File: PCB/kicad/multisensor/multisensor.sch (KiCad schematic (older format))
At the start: 27 parts

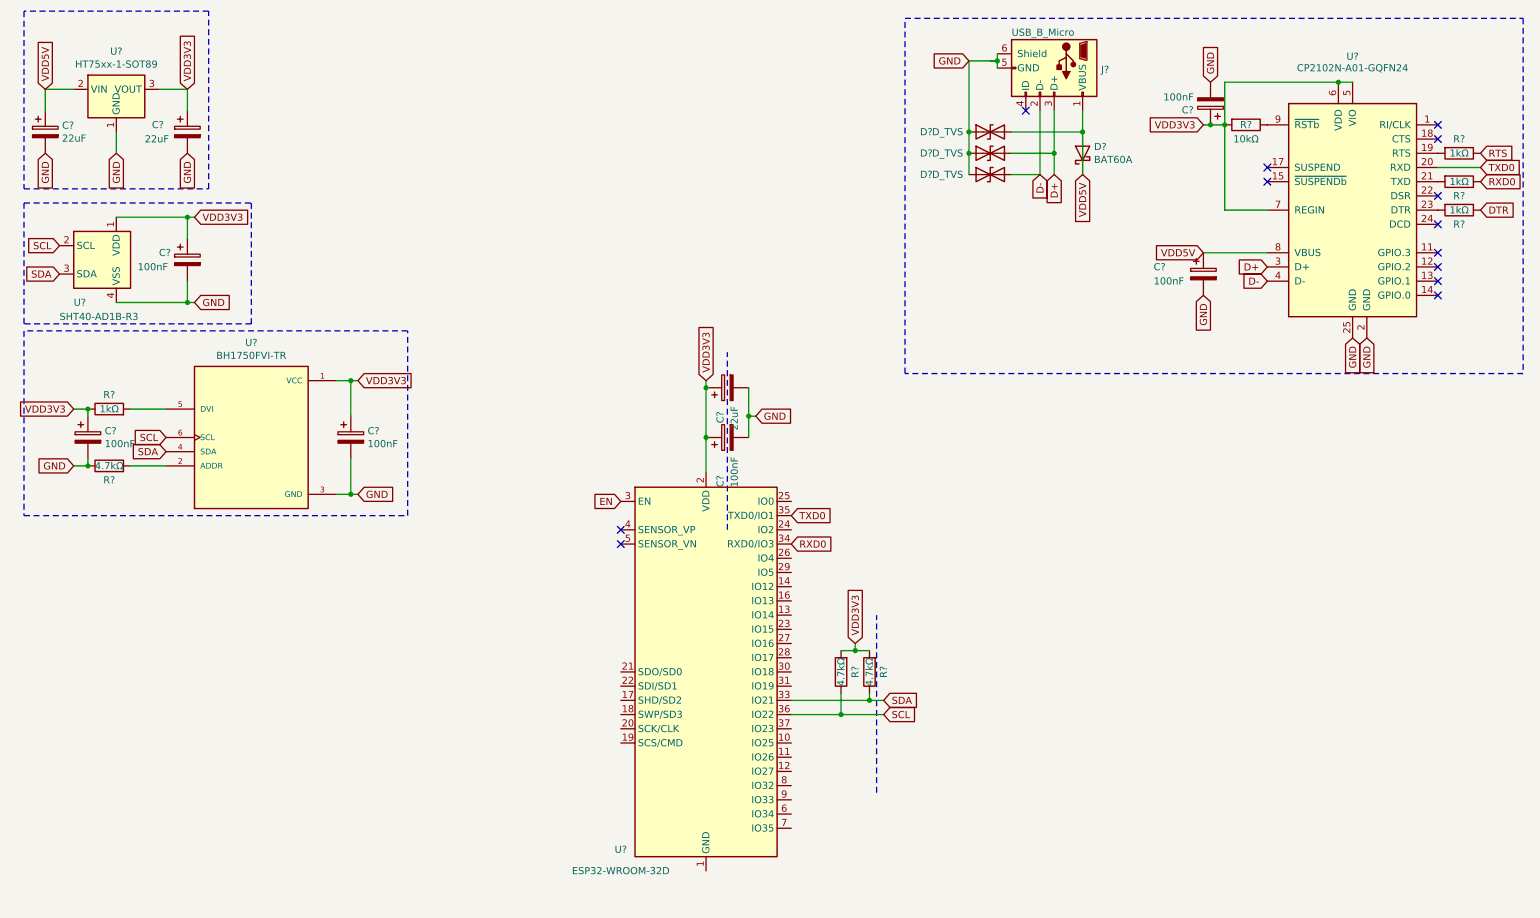
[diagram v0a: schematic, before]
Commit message: pogrammable part USB
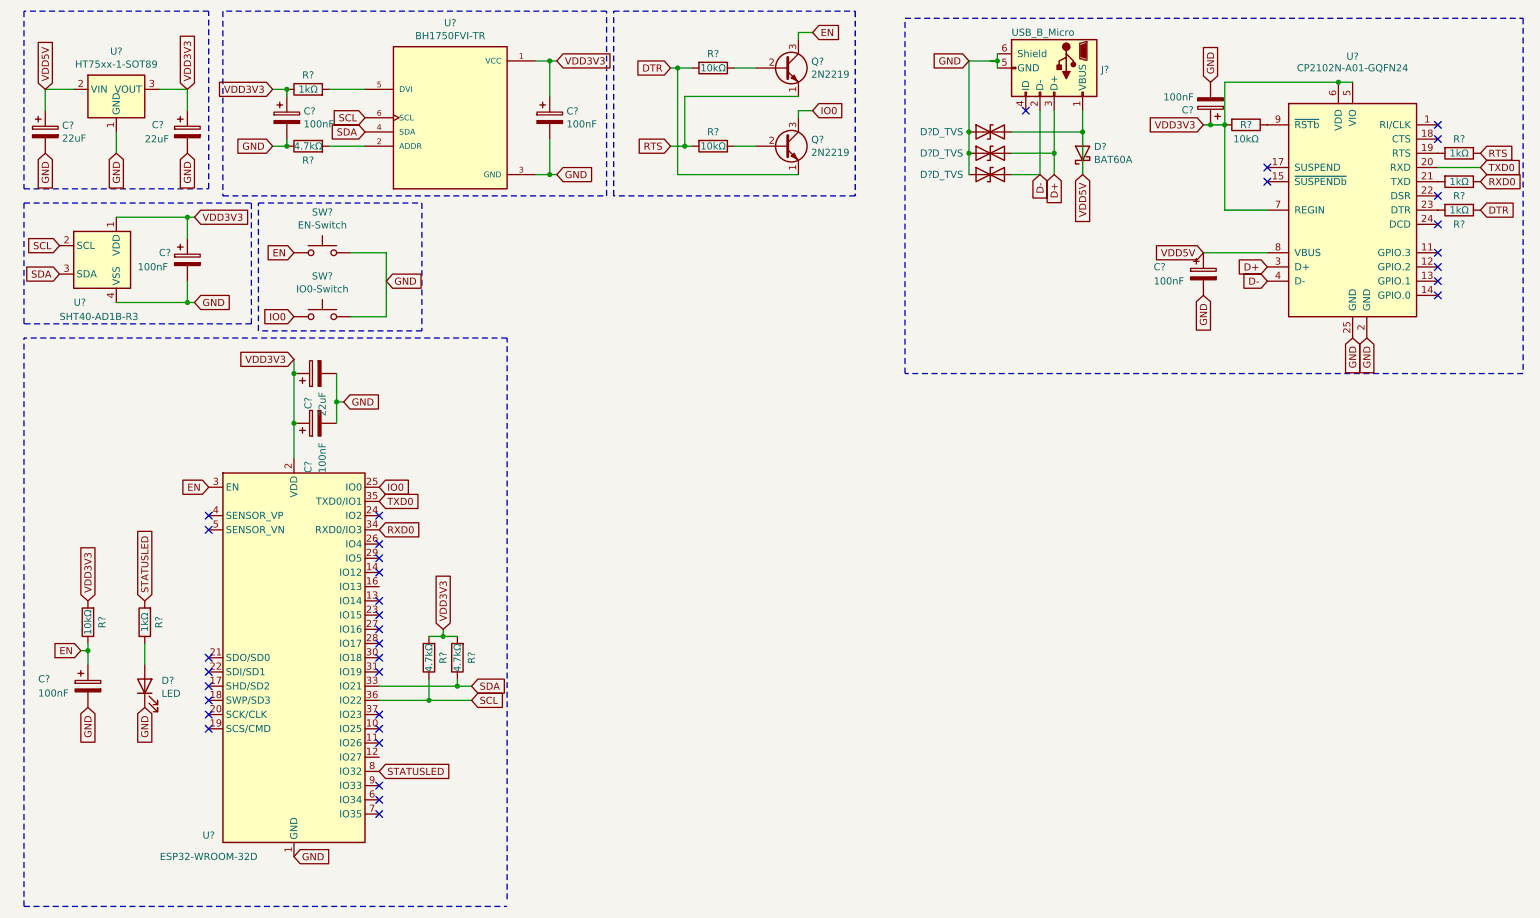
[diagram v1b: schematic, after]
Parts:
- added C?: 100nF, symbol Device:CP
- added D?: LED, symbol Device:LED
- added Q? (x2): 2N2219, Package_TO_SOT_THT:TO-39-3, symbol Transistor_BJT:2N2219
- added R? (x3): 10kΩ, symbol Device:R
- added R?: 1kΩ, symbol Device:R
- added SW?: EN-Switch, symbol Switch:SW_Push
- added SW?: IO0-Switch, symbol Switch:SW_Push
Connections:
- net DTR: now also Q?.1 (E), R?.2
- net EN: now also C?.1, Q?.3 (C), R?.1, SW?.1
- net GND: now also U?.1 (GND), U?.15 (GND), U?.38 (GND), U?.39 (GND), C?.2, D?.1 (K), SW?.2, SW?.2
- net RTS: now also Q?.1 (E), R?.2
- net VDD3V3: now also R?.2
- net IO0: now reaches U?.25 (IO0)
- net IO0: now also Q?.3 (C), SW?.1
- net STATUSLED: now reaches U?.8 (IO32)
- net STATUSLED: now also R?.2
- new net: D?.2 (A), R?.1
- new net: Q?.2 (B), R?.1 (x2)
- no-connect marks 13 -> 35
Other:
- moved on the sheet: C?, R?, U?
